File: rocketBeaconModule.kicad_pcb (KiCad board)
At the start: 2 copper layers, 80.5 x 49.3 mm, 72 parts, among them J1 TYPE-C-31-M-12, J2 MODE, J3 Main Bus, P1 AntMount, U1 STM32F401CCU6, U2 AMS1117-3.3, U3 CC1200, X1 40mhz, Y1 16MHz

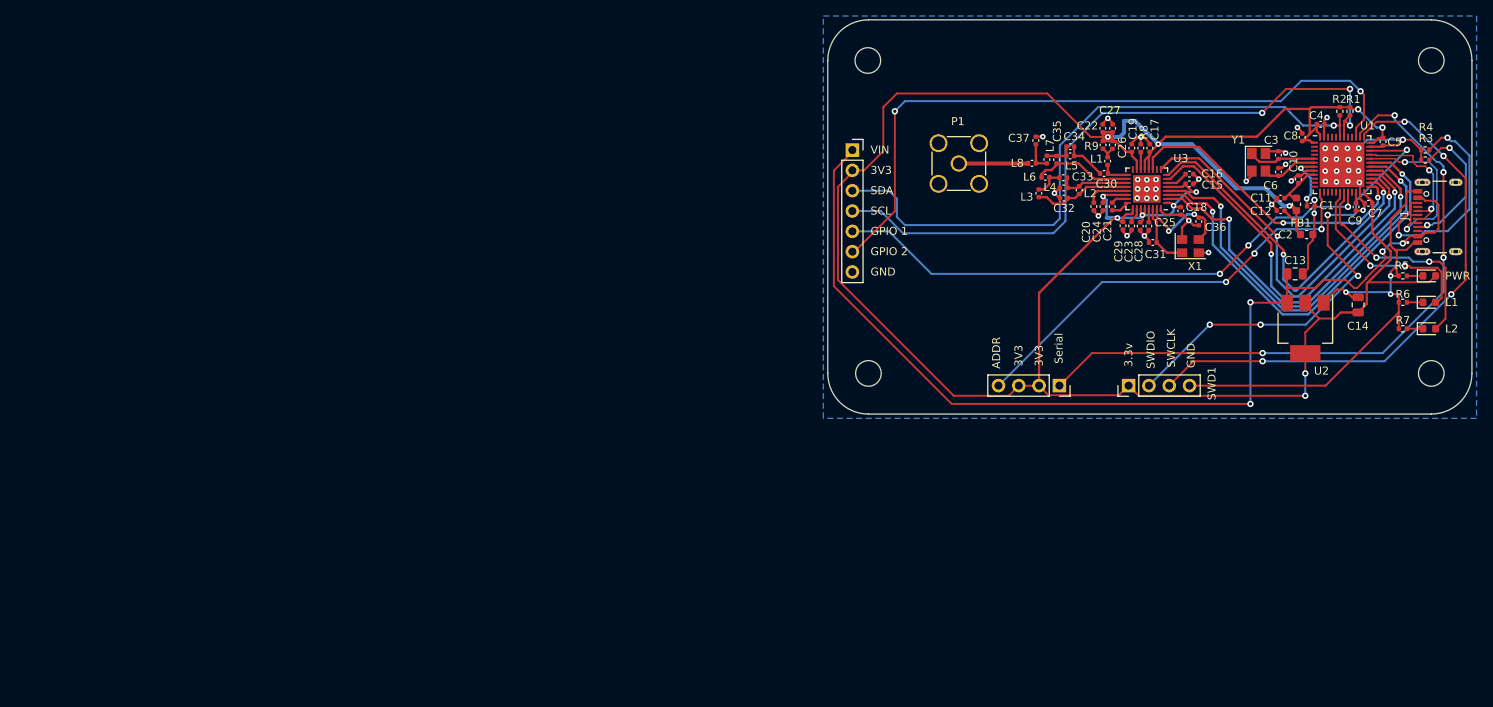
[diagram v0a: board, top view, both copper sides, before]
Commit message: V3 changes
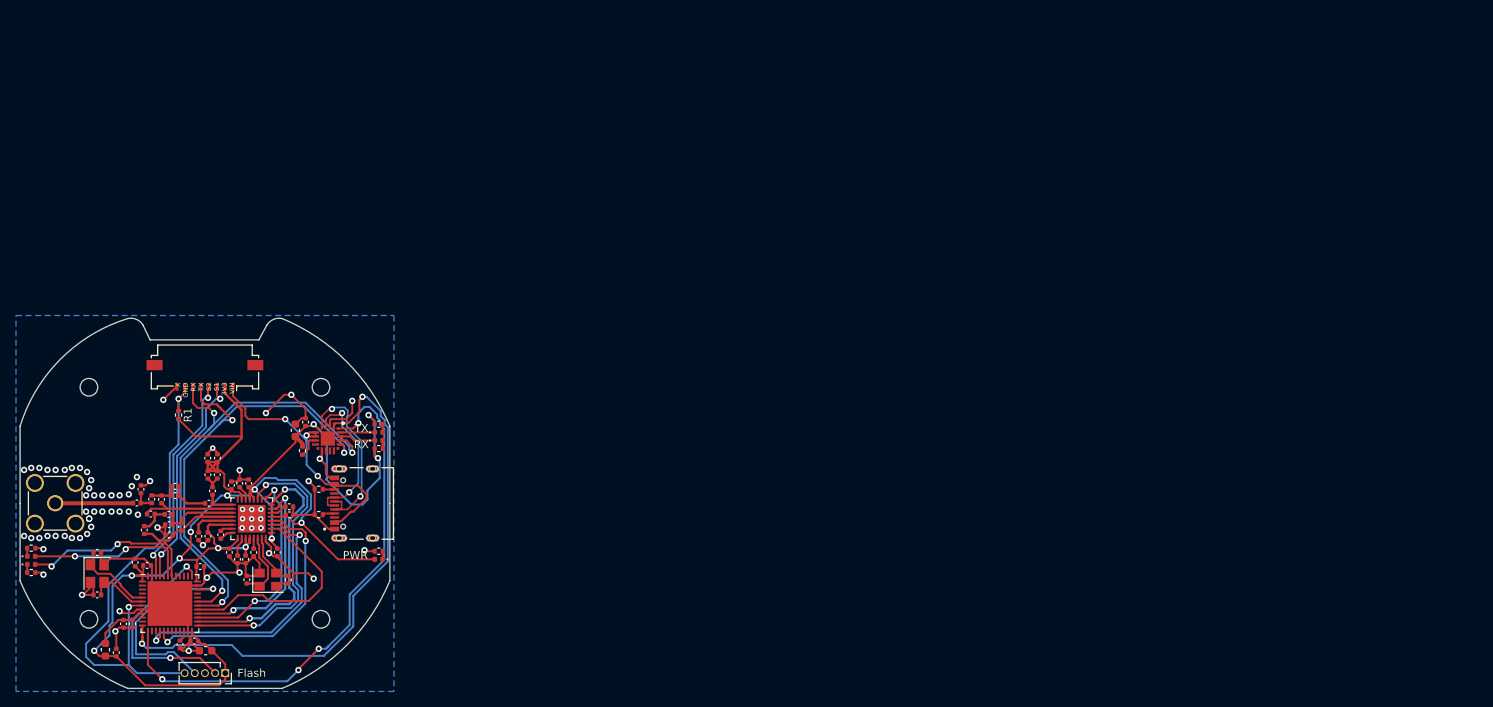
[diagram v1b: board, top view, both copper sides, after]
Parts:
- removed C14: 22u, Capacitor_SMD:C_0805_2012Metric
- removed J2: MODE, Connector_PinSocket_2.54mm:PinSocket_1x04_P2.54mm_Vertical
- removed J3: Main Bus, Connector_PinSocket_2.54mm:PinSocket_1x07_P2.54mm_Vertical
- removed R2: 1.5k, Resistor_SMD:R_0402_1005Metric
- added D4: TXT, LED_SMD:LED_0402_1005Metric, F.Cu at (93.7, 117.9)
- added D5: RXT, LED_SMD:LED_0402_1005Metric, F.Cu at (93.7, 118.9)
- added EX1: EXT1, Connector_FFC-FPC:Molex_200528-0080_1x08-1MP_P1.00mm_Horizontal, F.Cu at (72.0, 111.2)
- added R10: 1k, Resistor_SMD:R_0402_1005Metric, F.Cu at (93.7, 116.8)
- added R11: 1k, Resistor_SMD:R_0402_1005Metric, F.Cu at (93.7, 119.9)
- added R12: 5.11k, Resistor_SMD:R_0402_1005Metric, F.Cu at (84.2, 120.1)
- C1: value 100n -> 4.7uF; footprint Capacitor_SMD:C_0402_1005Metric -> Capacitor_SMD:C_0603_1608Metric
- C10: value 10n -> 10nF
- C11, C12: value 1u -> 1uF
- C13: value 22u -> 100nF; footprint Capacitor_SMD:C_0805_2012Metric -> Capacitor_SMD:C_0402_1005Metric
- C2: value 10u -> 10uF
- C3, C6: value 10p -> 10pF
- C4, C5, C7, C8: value 100n -> 100nF
- C9: value 2.2u -> 2.2uF
- D1: value LED -> PWR_LED; footprint LED_SMD:LED_0603_1608Metric -> LED_SMD:LED_0402_1005Metric
- D2, D3: footprint LED_SMD:LED_0603_1608Metric -> LED_SMD:LED_0402_1005Metric
- H1, H2, H3, H4: footprint MountingHole:MountingHole_3.2mm_M3 -> MountingHole:MountingHole_2.2mm_M2
- R1: value 1.5k -> 5.11k
- R9: value 18 -> 18k
- SWD1: footprint Connector_PinHeader_2.54mm:PinHeader_1x04_P2.54mm_Vertical -> Connector_PinSocket_1.27mm:PinSocket_1x05_P1.27mm_Vertical
- U2: value AMS1117-3.3 -> CP2102N-Axx-xQFN20; footprint Package_TO_SOT_SMD:SOT-223-3_TabPin2 -> CP2102:WFQFN-20
- X1: value 40mhz -> 40MHz
- moved H3 181.8 mm to (57.5, 141.2)
- moved D2 177.6 mm to (50.3, 133.3)
- moved D3 177.2 mm to (50.3, 134.4)
- moved R6 174.2 mm to (50.3, 132.3), turned to 0 degrees
- moved R7 174.1 mm to (50.3, 135.4), turned to 0 degrees
- moved C5 163.3 mm to (64.8, 134.5), turned to 0 degrees
- moved C7 160.6 mm to (63.3, 134.1), turned to 90 degrees
- moved FB1 159.0 mm to (59.6, 145.0)
- moved C9 156.8 mm to (68.9, 144.4)
- moved C6 156.8 mm to (58.5, 138.2), turned to 180 degrees
- moved U1 156.4 mm to (67.6, 139.3)
- moved C10 156.0 mm to (62.9, 141.8), turned to -90 degrees
- moved C3 155.8 mm to (58.5, 132.9), turned to 0 degrees
- moved C12 155.7 mm to (60.9, 145.4), turned to 90 degrees
- moved C4 154.9 mm to (70.7, 144.0), turned to 180 degrees
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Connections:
- net /PWR_LED_K renamed Net-(D1-Pad1)
- C1 pad 1: /NRST -> +3.3V
- C13 pad 1: VBUS -> +3.3V
- J1 pad A6: /USB_D+ -> /D+
- J1 pad A7: /USB_D- -> /D-
- J1 pad B6: /USB_D+ -> /D+
- J1 pad B7: /USB_D- -> /D-
- J1 pad S1: unconnected-(J1-PadS1) -> GND
- J1 pad S2: unconnected-(J1-PadS2) -> GND
- J1 pad S3: unconnected-(J1-PadS3) -> GND
- J1 pad S4: unconnected-(J1-PadS4) -> GND
- R1 pad 1: +3.3V -> /NRST
- R1 pad 2: /I2C_SCL -> +3.3V
- SWD1 pad 2: /SWDIO -> /SWCLK
- SWD1 pad 3: /SWCLK -> GND
- SWD1 pad 4: GND -> /SWDIO
- U1 pad 12: unconnected-(U1-Pad12) -> /CP2102N_SIG1
- U1 pad 13: /ADDR -> /CP2102N_SIG2
- U1 pad 16: unconnected-(U1-Pad16) -> RADIO_MARC_INT
- U1 pad 17: unconnected-(U1-Pad17) -> RADIO_INT
- U1 pad 18: /LED1 -> unconnected-(U1-Pad18)
- U1 pad 19: /LED2 -> unconnected-(U1-Pad19)
- U1 pad 20: /GPIO1 -> unconnected-(U1-Pad20)
- U1 pad 30: RADIO_INT -> /TX
- U1 pad 31: RADIO_MARC_INT -> /RX
- U1 pad 32: /USB_D- -> unconnected-(U1-Pad32)
- U1 pad 33: /USB_D+ -> unconnected-(U1-Pad33)
- U1 pad 38: /Serial -> unconnected-(U1-Pad38)
- U1 pad 39: /GPIO2 -> unconnected-(U1-Pad39)
- U1 pad 42: /I2C_SCL -> /LED2
- U1 pad 43: /I2C_SDA -> /LED1
- U1 pad 45: unconnected-(U1-Pad45) -> /S1
- U1 pad 46: unconnected-(U1-Pad46) -> /S2
- U2 pad 1: GND -> /CP2102N_SIG2
- U2 pad 2: +3.3V -> /CP2102N_SIG1
- U2 pad 3: VBUS -> GND
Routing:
- net +3.3V: track 323.7 -> 212.1 mm, vias 12 -> 13
- net VBUS: track 127.2 -> 35.1 mm, vias 4 -> 3
- net /GPIO2: track 86.2 -> 0.00 mm, vias 2 -> 0
- net /I2C_SCL: track 84.4 -> 0.00 mm, vias 3 -> 0
- net /Serial: track 83.4 -> 0.00 mm, vias 4 -> 0
- net /I2C_SDA: track 79.0 -> 0.00 mm, vias 1 -> 0
- net /CP2102N_SIG1: track 0.00 -> 70.0 mm, vias 0 -> 2
- net /CP2102N_SIG2: track 0.00 -> 69.4 mm, vias 0 -> 4
- net /GPIO1: track 69.2 -> 0.00 mm, vias 3 -> 0
- net /TX: track 0.00 -> 59.7 mm, vias 0 -> 3
- net /RX: track 0.00 -> 59.7 mm, vias 0 -> 3
- net /NRST: track 7.27 -> 63.3 mm
- net /ADDR: track 53.3 -> 0.00 mm, vias 3 -> 0
- net /SWCLK: track 71.9 -> 26.8 mm, vias 4 -> 2
- net /SWDIO: track 59.9 -> 25.9 mm, vias 5 -> 1
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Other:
- board size 80.5 x 49.3 mm -> 46.2 x 46.3 mm
- board text added: "50mm"
- board text added: "ArmstrongLabs"
- board text added: "Flash"
- board text added: "RX"
- board text added: "SubGhz Transciever"
- board text added: "TX"
- board text added: "V3"
- board text added: "X GND RX TX S2 S1 3V3 VIN"
- board text removed: "3.3v"
- board text removed: "3V3"
- board text removed: "ADDR"
- board text removed: "Armstrong Labs"
- board text removed: "CC1200 Radio Module"
- board text removed: "GND"
- board text removed: "GPIO 1"
- board text removed: "GPIO 2"
- board text removed: "L1"
- board text removed: "L2"
- board text removed: "SCL"
- board text removed: "SDA"
- board text removed: "SWCLK"
- board text removed: "SWDIO"
- board text removed: "Serial"
- board text removed: "VIN"
- board text removed: "v1.1"
